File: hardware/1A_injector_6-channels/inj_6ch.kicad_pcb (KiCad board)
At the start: 2 copper layers, 47.6 x 36.2 mm, 35 parts, among them P1 CONN_10X2, P2 CONN_2, P3 CONN_3, P4 CONN_2, P5 CONN_3, P7 CONN_10X2, Q1 OVP_DRIVER, Q2 OVP_DRIVER, Q3 OVP_DRIVER, Q4 OVP_DRIVER, Q5 OVP_DRIVER, Q6 OVP_DRIVER

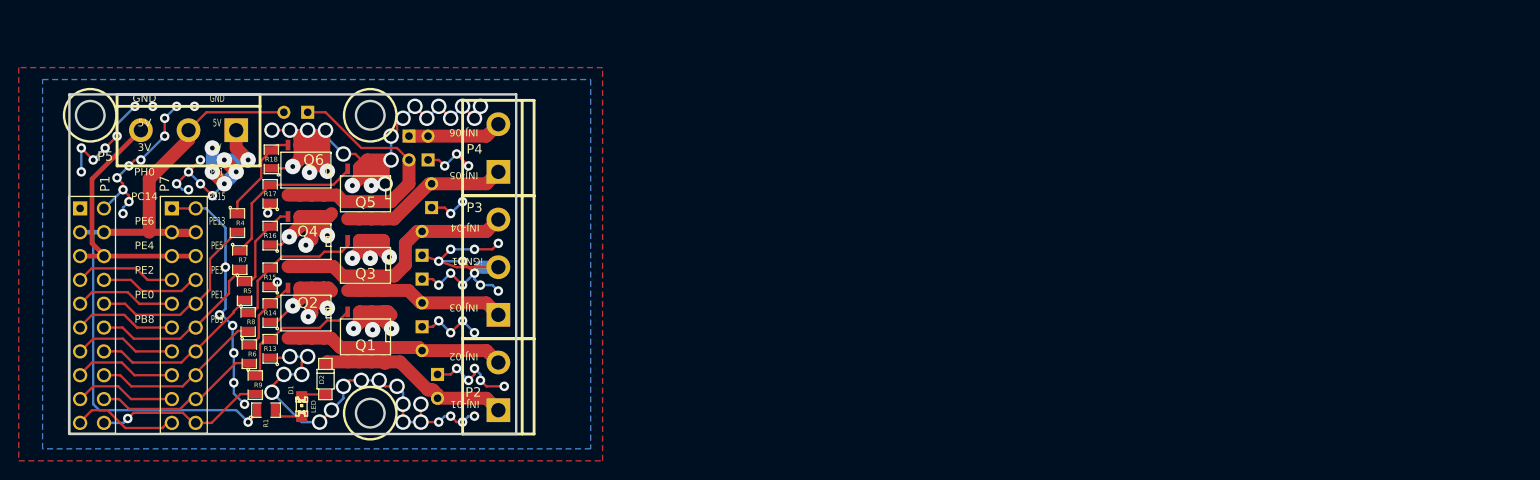
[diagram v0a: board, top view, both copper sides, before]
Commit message: getting ready for Frankenstein
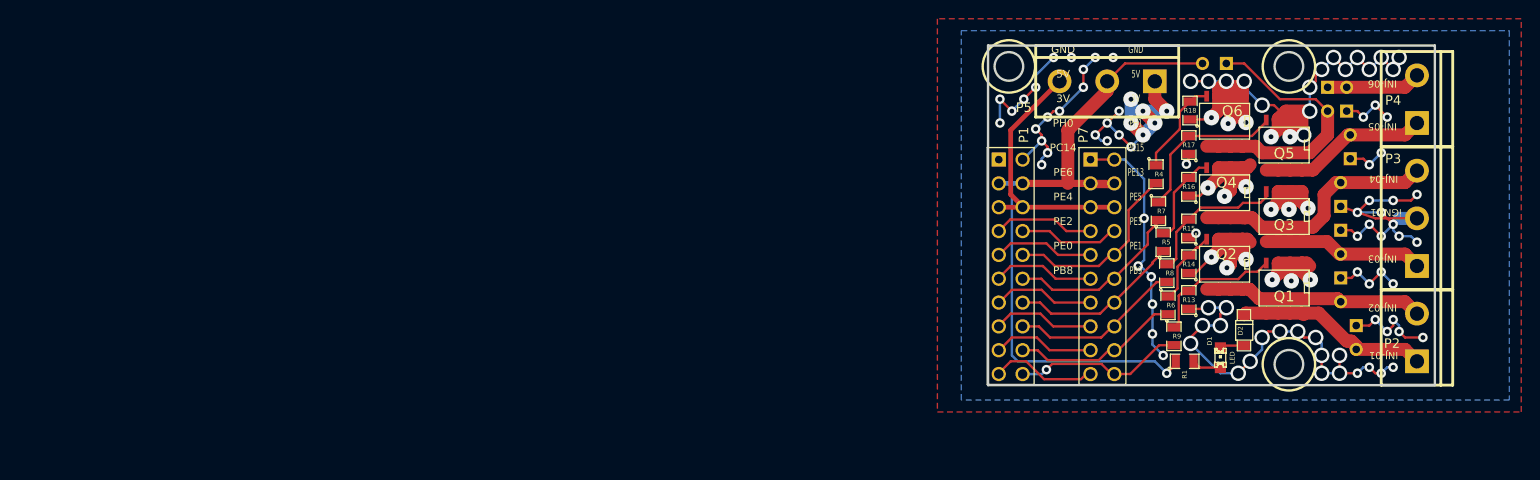
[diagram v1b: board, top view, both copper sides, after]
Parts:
- moved P2 98.1 mm to (222.4, 145.9)
- moved P3 98.1 mm to (222.4, 133.2)
- moved P4 98.1 mm to (222.4, 120.5)
- moved R18 98.1 mm to (198.2, 121.7)
- moved R7 98.1 mm to (194.8, 132.5)
- moved D1 98.1 mm to (201.4, 148.1)
- moved D4 98.1 mm to (214.2, 130.7)
- moved D5 98.1 mm to (214.2, 140.8)
- moved D7 98.1 mm to (214.2, 135.8)
- moved D8 98.1 mm to (215.9, 145.9)
- moved P5 98.1 mm to (189.4, 118.6)
- moved Q1 98.1 mm to (208.2, 140.7)
- moved Q2 98.1 mm to (201.9, 138.1)
- moved Q3 98.1 mm to (208.2, 133.0)
- moved Q4 98.1 mm to (201.9, 130.5)
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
